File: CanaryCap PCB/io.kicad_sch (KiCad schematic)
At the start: 20 parts, among them J1 USB_C_Receptacle_USB2.0_16P, J2 Impact Connector, J3 Gas Connector, J4 Battery Connector, Q1 NMOS, Q2 PMOS_Substrate, U4 ADXL343

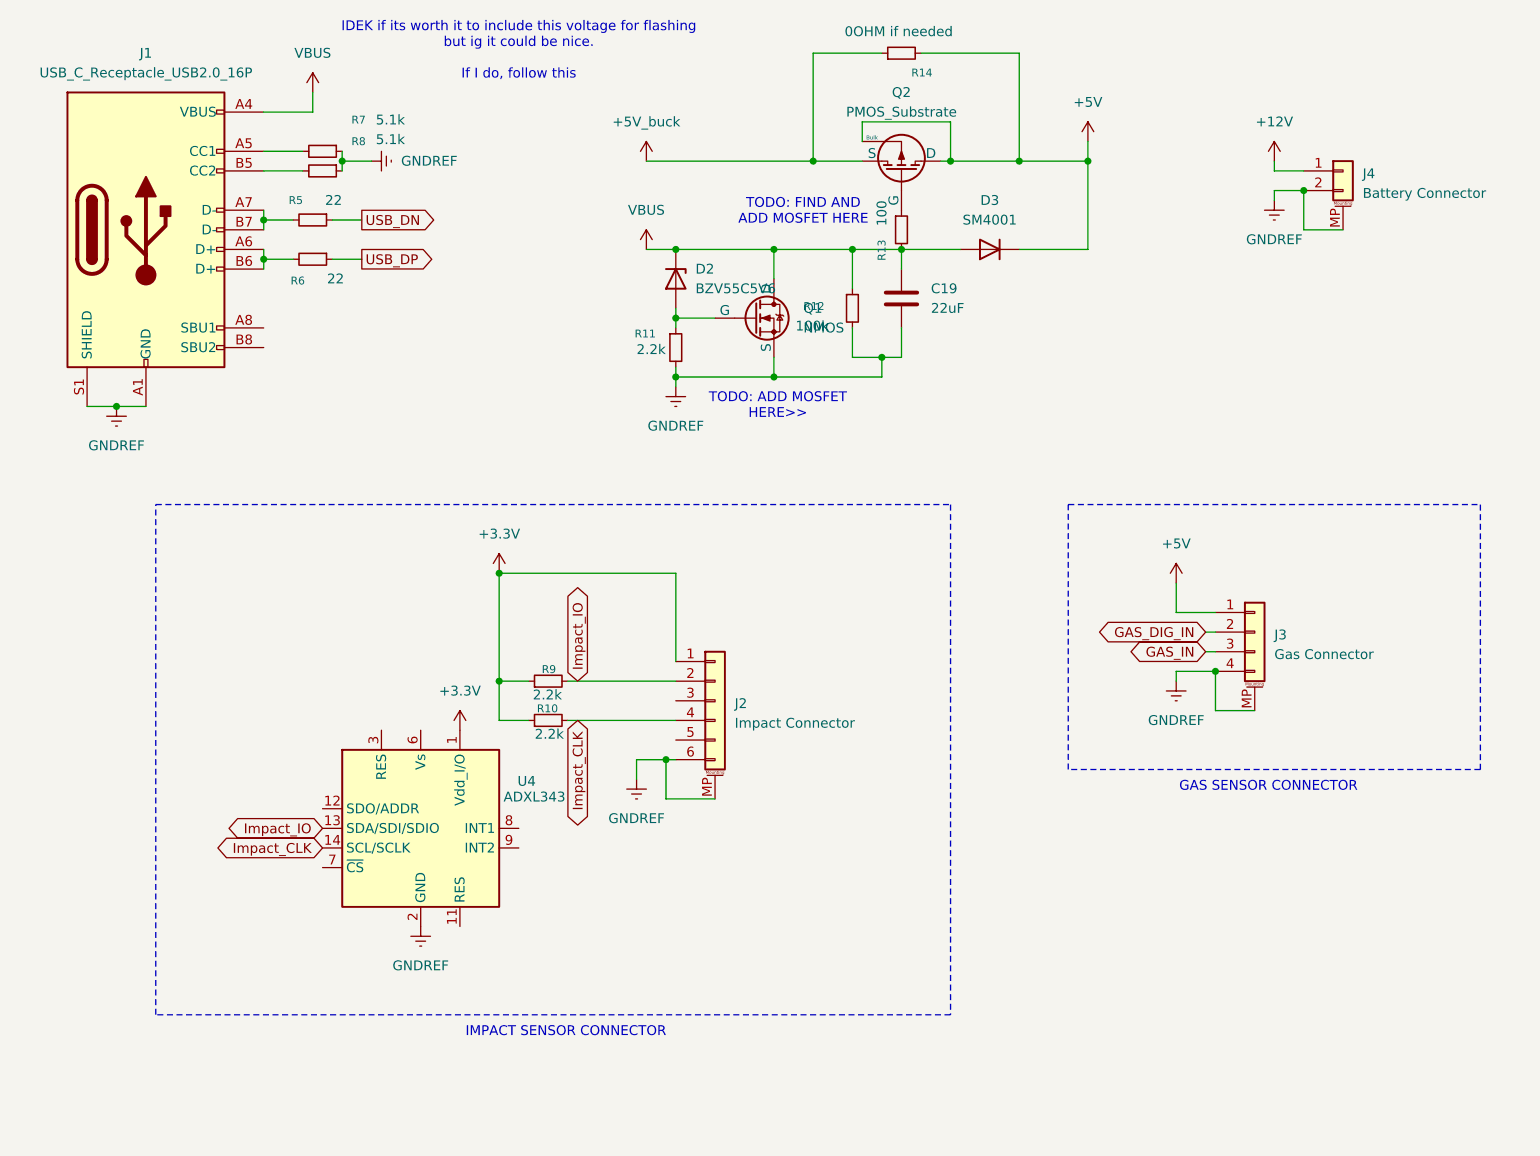
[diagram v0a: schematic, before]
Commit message: YIPPEE
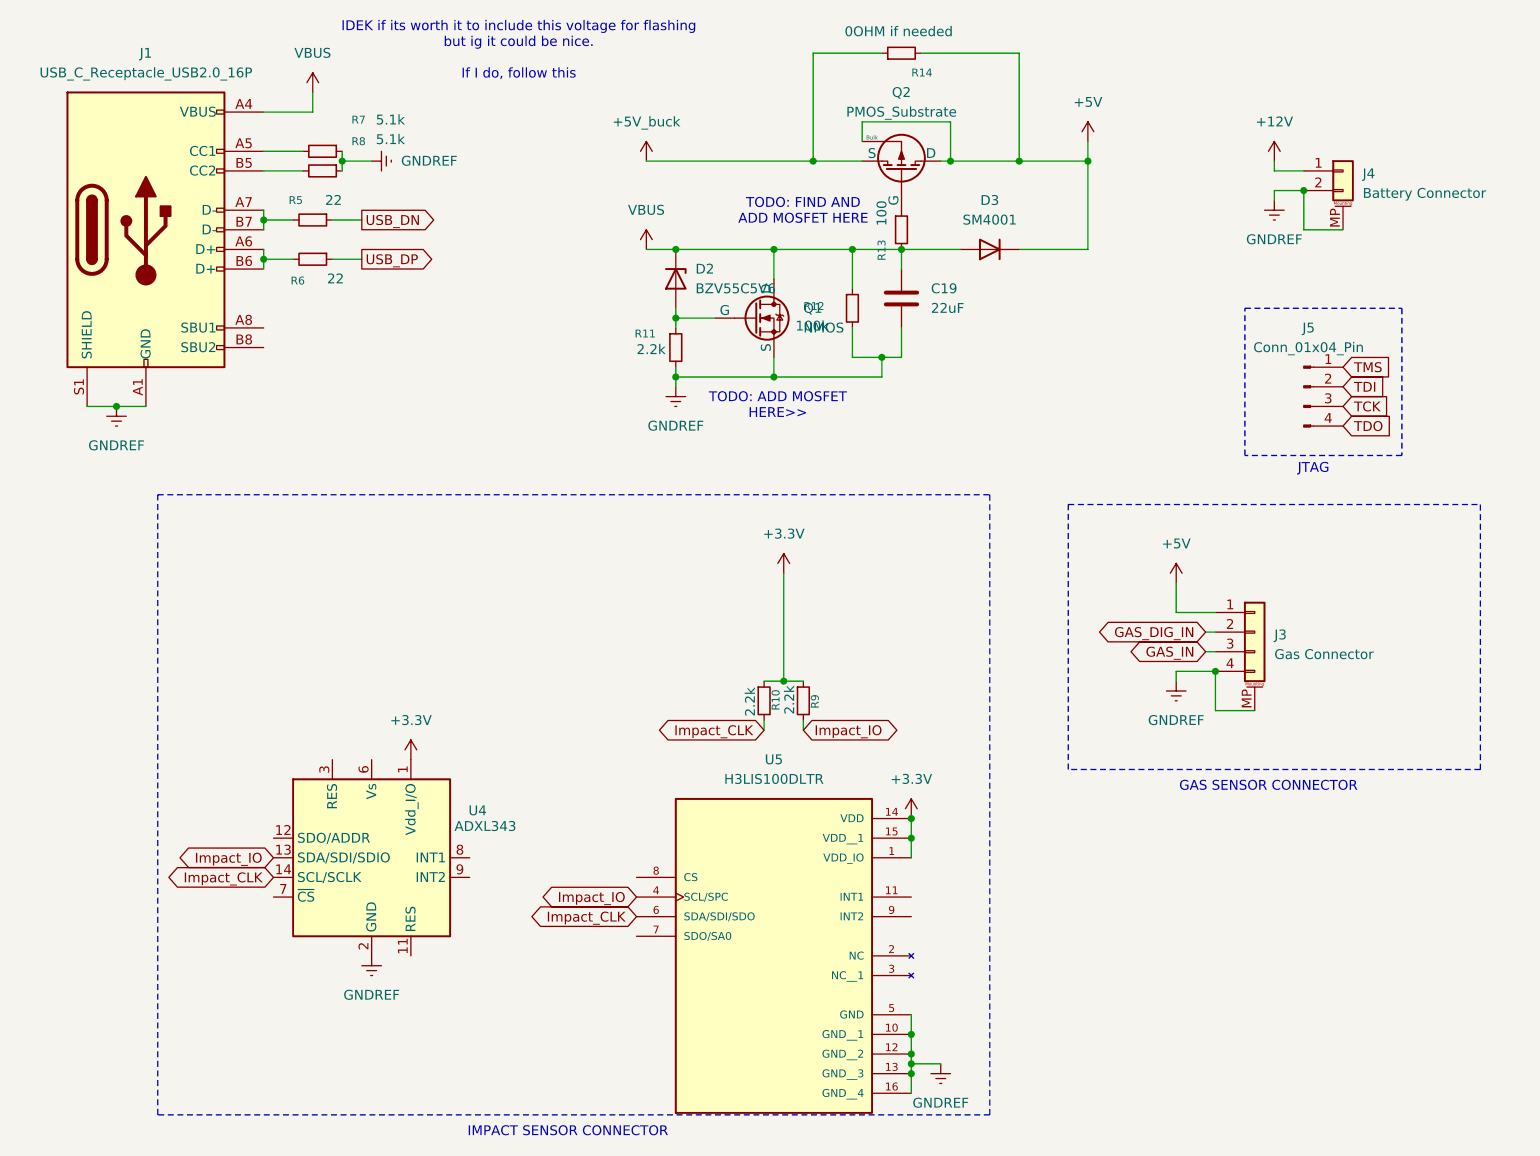
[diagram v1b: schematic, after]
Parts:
- removed J2: Impact Connector, Connector_Molex:Molex_CLIK-Mate_502443-0670_1x06-1MP_P2.00mm_Vertical, symbol Connector_Generic_MountingPin:Conn_01x06_MountingPin
- added J5: Conn_01x04_Pin, Connector_PinHeader_2.54mm:PinHeader_1x04_P2.54mm_Vertical, symbol Connector:Conn_01x04_Pin
- added U5: H3LIS100DLTR, Library:H3LIS100DLTR, symbol ESP-32-C6:H3LIS100DLTR
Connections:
- net +3.3V: now also U5.1 (VDD_IO), U5.14 (VDD), U5.15 (VDD__1)
- net GNDREF: now also U5.10 (GND__1), U5.12 (GND__2), U5.13 (GND__3), U5.16 (GND__4), U5.5 (GND)
- net Impact_CLK: now also U5.6 (SDA/SDI/SDO)
- net Impact_IO: now also U5.4 (SCL/SPC)
- new net TCK: J5.3 (Pin_3)
- new net TDI: J5.2 (Pin_2)
- new net TDO: J5.4 (Pin_4)
- new net TMS: J5.1 (Pin_1)
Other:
- note added: "JTAG"
- moved on the sheet: R10, R9, U4

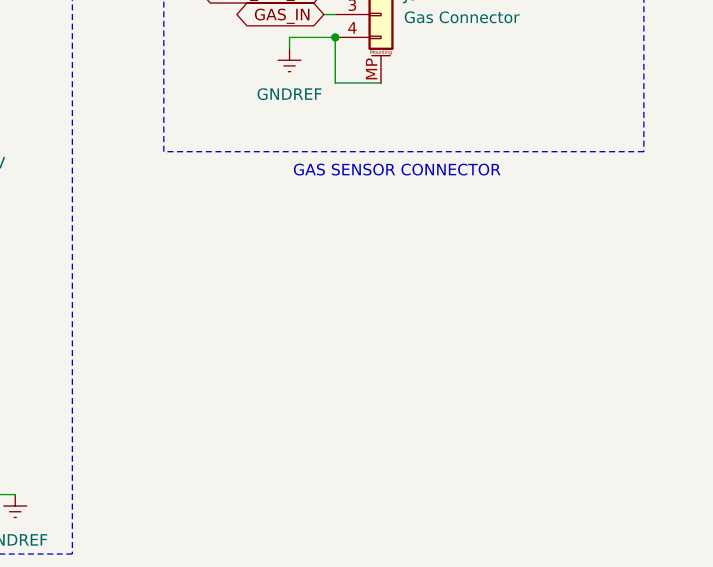
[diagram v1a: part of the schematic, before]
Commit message: Bruh
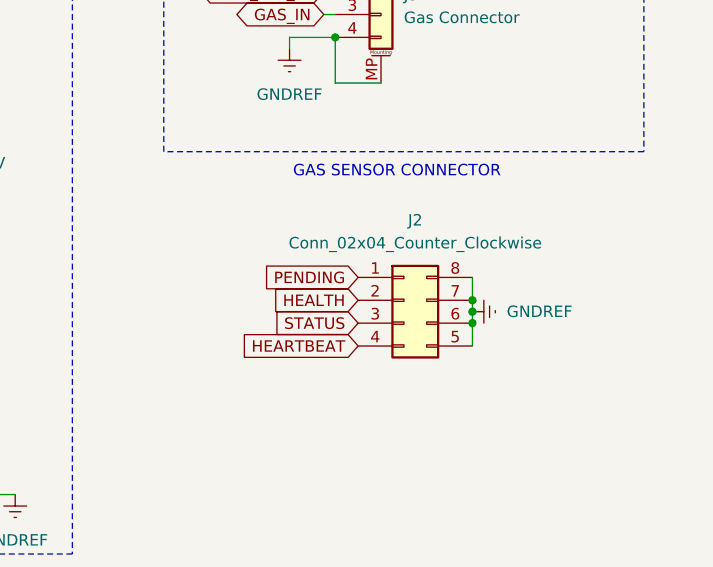
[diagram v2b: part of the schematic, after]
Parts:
- added J2: Conn_02x04_Counter_Clockwise, Connector_Harwin:Harwin_LTek-Male_2x04_P2.00mm_Vertical, symbol Connector_Generic:Conn_02x04_Counter_Clockwise
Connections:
- net GNDREF: now also J2.5 (Pin_5), J2.6 (Pin_6), J2.7 (Pin_7), J2.8 (Pin_8)
- new net HEALTH: J2.2 (Pin_2)
- new net HEARTBEAT: J2.4 (Pin_4)
- new net PENDING: J2.1 (Pin_1)
- new net STATUS: J2.3 (Pin_3)

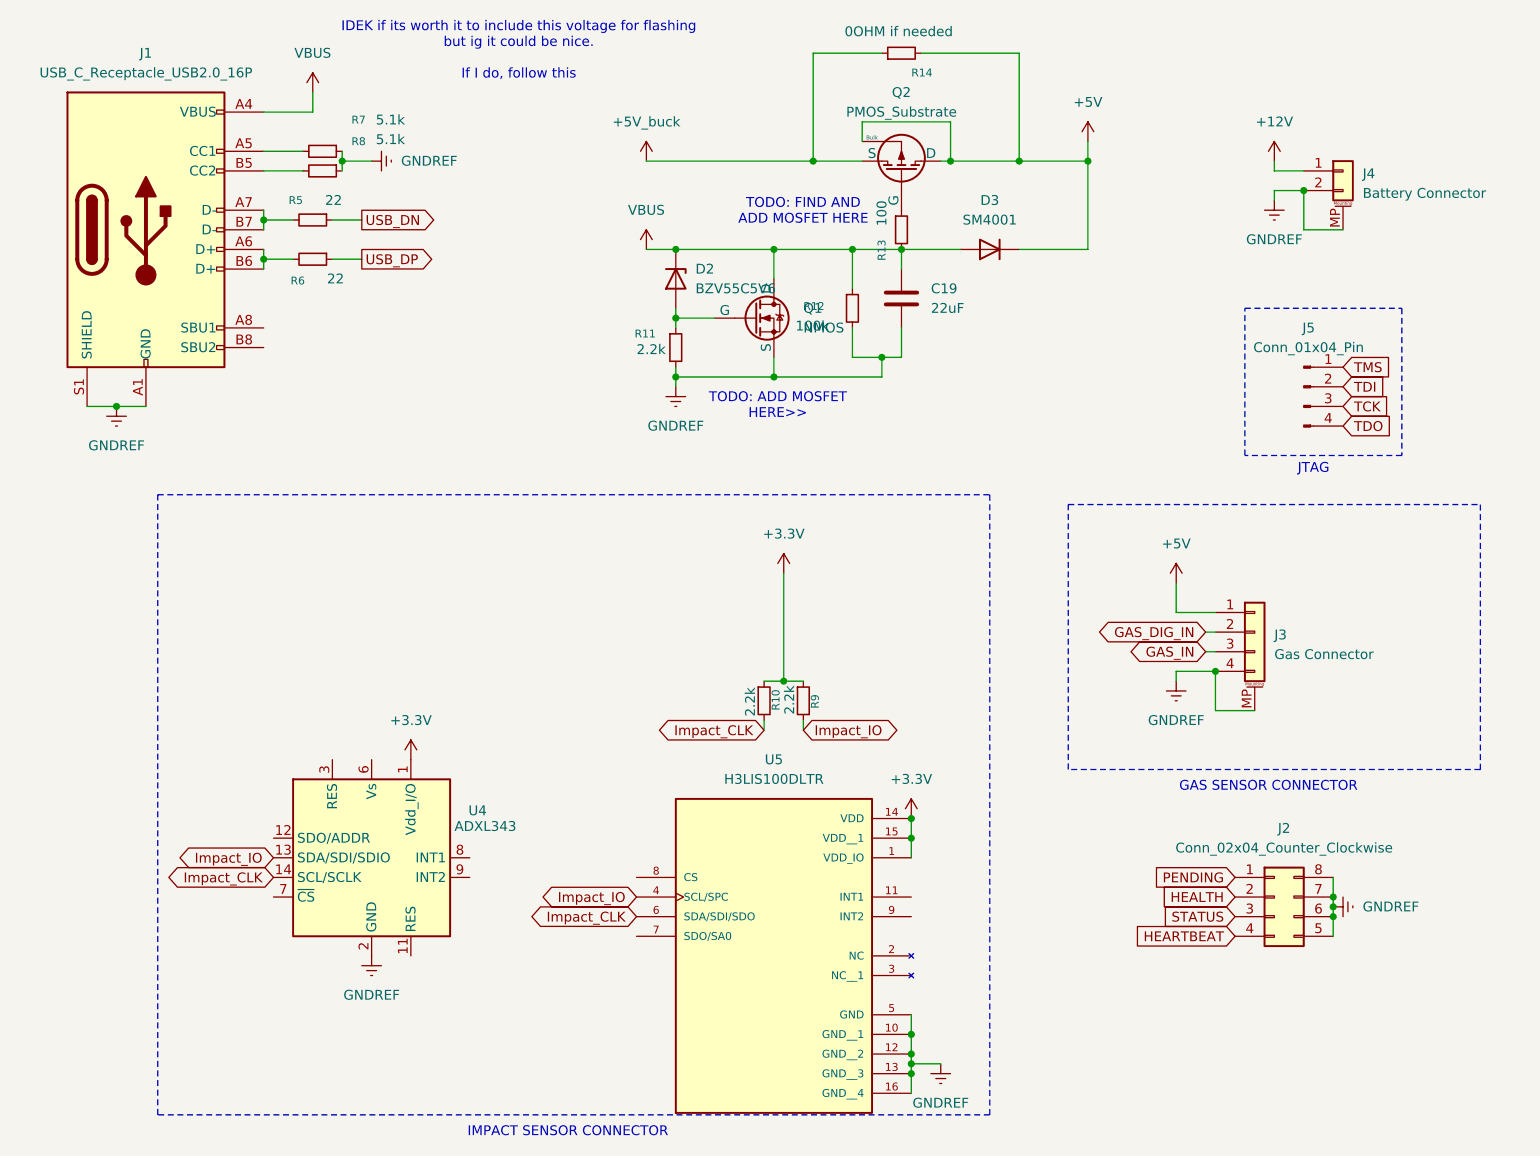
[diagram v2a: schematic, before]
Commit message: Capcb updates
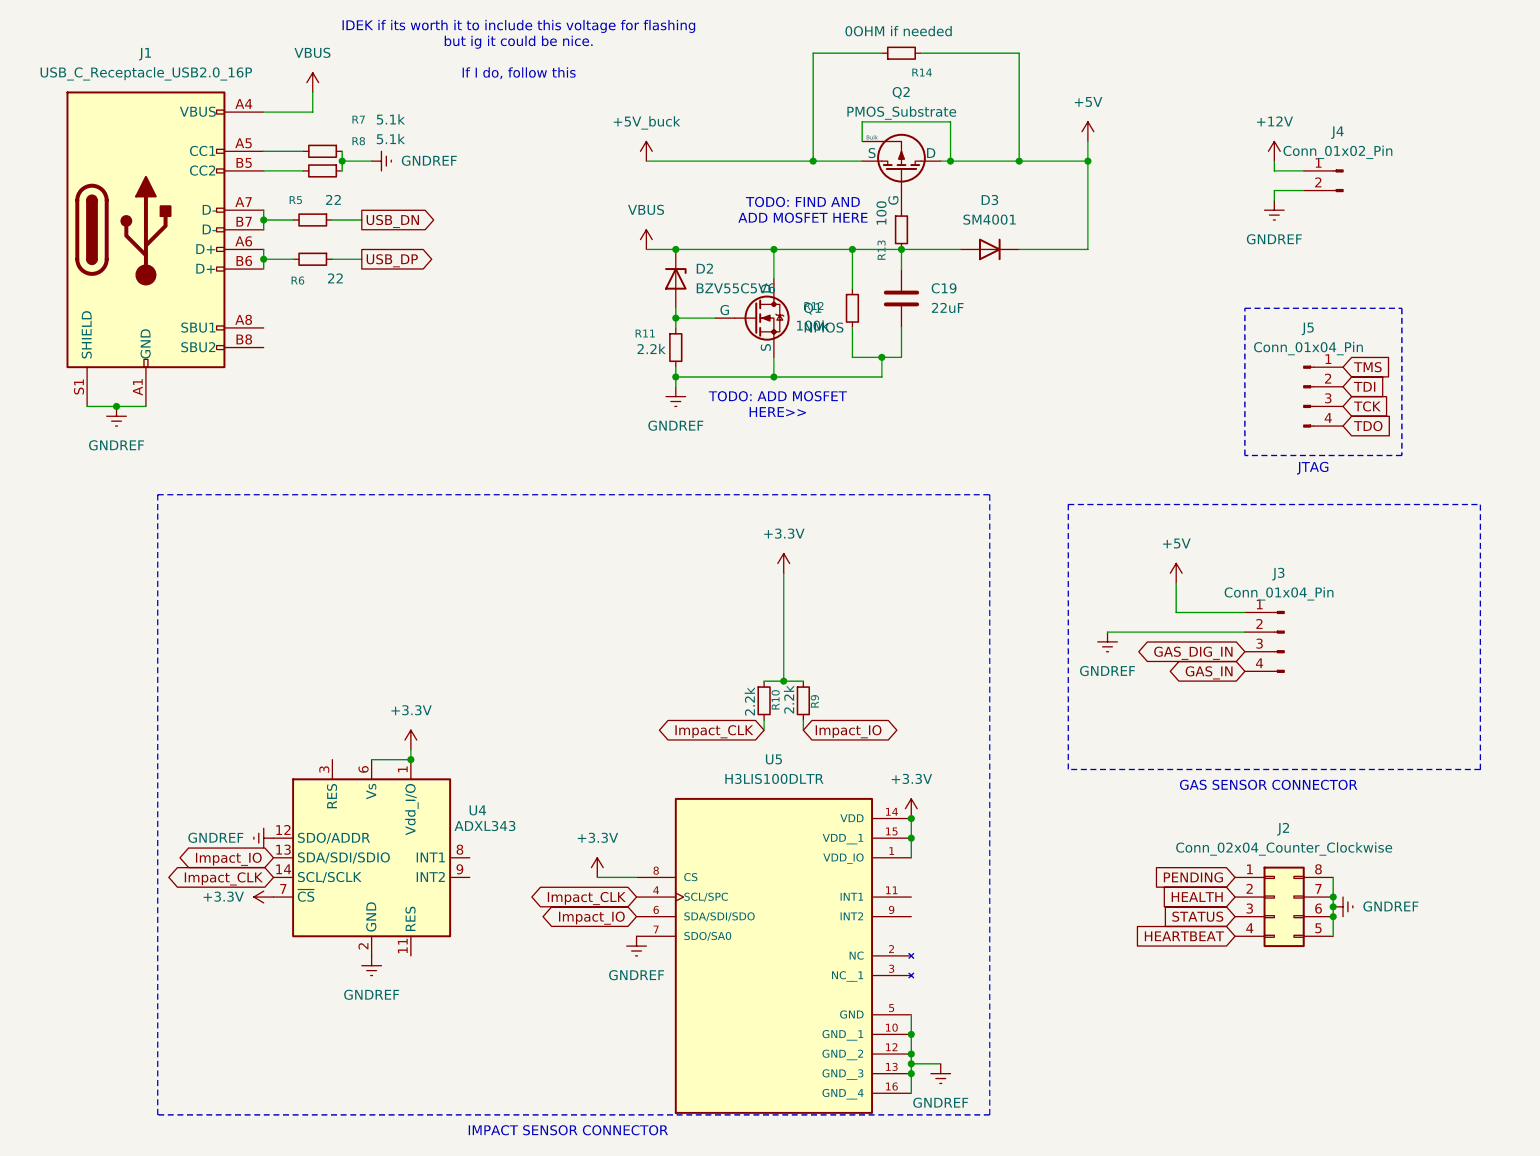
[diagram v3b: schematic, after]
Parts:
- removed J3: Gas Connector, Connector_Molex:Molex_CLIK-Mate_502443-0470_1x04-1MP_P2.00mm_Vertical, symbol Connector_Generic_MountingPin:Conn_01x04_MountingPin
- removed J4: Battery Connector, Connector_Molex:Molex_CLIK-Mate_502443-0270_1x02-1MP_P2.00mm_Vertical, symbol Connector_Generic_MountingPin:Conn_01x02_MountingPin
- added J3: Conn_01x04_Pin, Connector_PinHeader_2.54mm:PinHeader_1x04_P2.54mm_Vertical, symbol Connector:Conn_01x04_Pin
- added J4: Conn_01x02_Pin, Connector_PinHeader_2.54mm:PinHeader_1x02_P2.54mm_Vertical, symbol Connector:Conn_01x02_Pin
- J2: footprint Connector_Harwin:Harwin_LTek-Male_2x04_P2.00mm_Vertical -> Connector_PinHeader_2.54mm:PinHeader_2x04_P2.54mm_Vertical
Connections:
- net +12V: now also J4.1 (Pin_1)
- net +3.3V: now also U4.6 (Vs), U4.7 (~{CS}), U5.8 (CS)
- net +5V: now also J3.1 (Pin_1)
- net GAS_DIG_IN: now also J3.3 (Pin_3)
- net GAS_IN: now also J3.4 (Pin_4)
- net GNDREF: now also U4.12 (SDO/ADDR), U5.7 (SDO/SA0), J3.2 (Pin_2), J4.2 (Pin_2)
- net Impact_CLK: now also U5.4 (SCL/SPC); no longer U5.6 (SDA/SDI/SDO)
- net Impact_IO: now also U5.6 (SDA/SDI/SDO); no longer U5.4 (SCL/SPC)
